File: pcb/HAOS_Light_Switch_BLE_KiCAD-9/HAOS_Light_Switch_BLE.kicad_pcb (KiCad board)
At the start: 2 copper layers, 30.1 x 29.9 mm, 38 parts, among them J1 GPIO, J2 GPIO, J3 GPIO, J4 Battery_CR2032, J5 PWR, J6 Conn_ARM_SWD_TagConnect_TC203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, J7 SWD, SW1 SW_Push, SW2 SW_Push, SW3 SW_Push, U1 nrf52832, Y1 Q13FC1350000400, Y3 ABM8-32.000MHZ-B2-T3

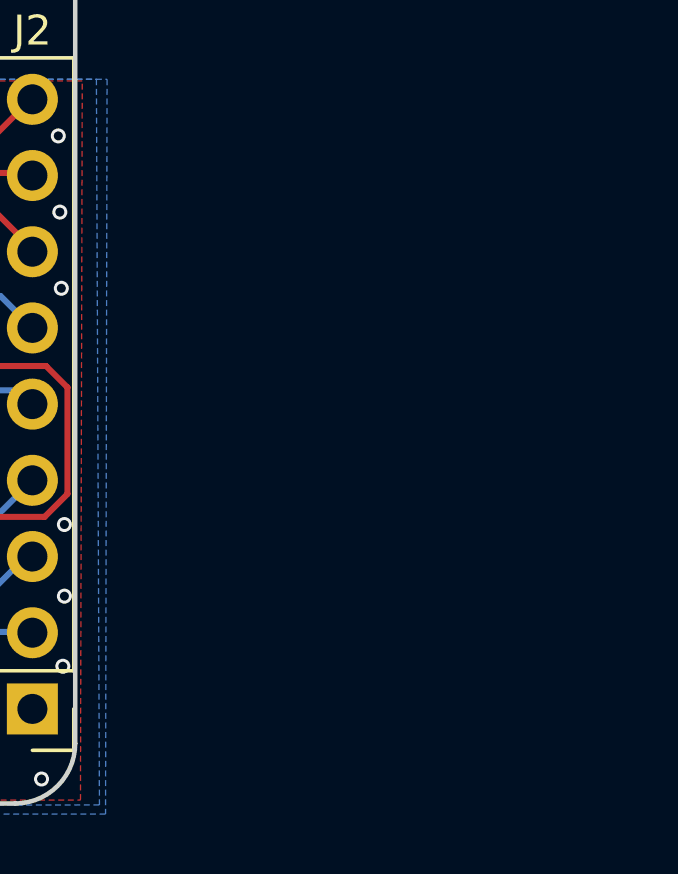
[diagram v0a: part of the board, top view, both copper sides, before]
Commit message: Draft AC power sniffer
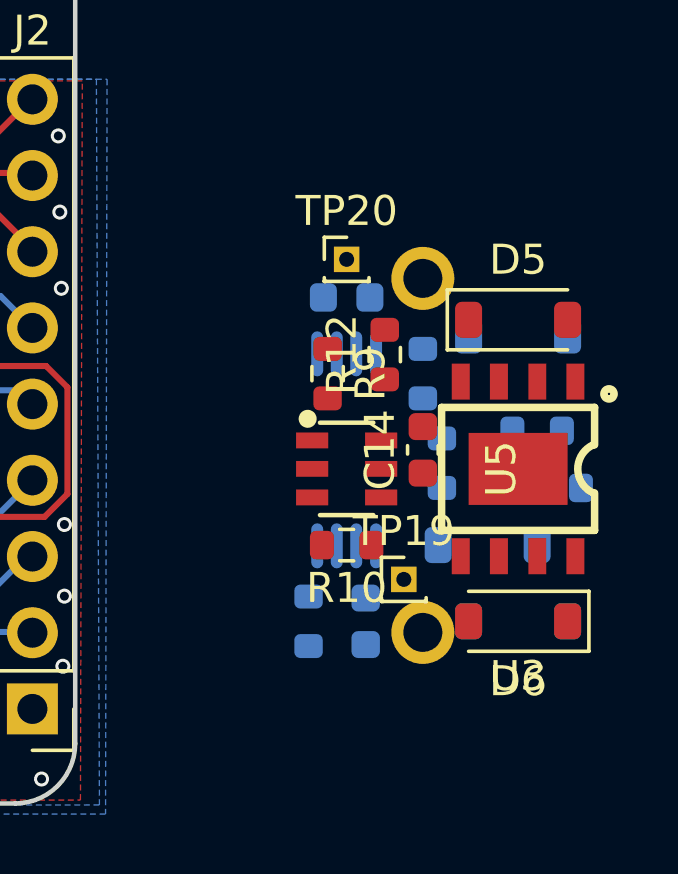
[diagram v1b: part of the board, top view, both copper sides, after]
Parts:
- added C14: 100n, Capacitor_SMD:C_0603_1608Metric, F.Cu at (205.1, 122.5)
- added C15: 10u, Capacitor_SMD:C_0603_1608Metric, B.Cu at (203.2, 128.2)
- added C16: 100n, Capacitor_SMD:C_0603_1608Metric, B.Cu at (202.6, 117.5)
- added D4: MBR0530, Diode_SMD:D_SOD-123, B.Cu at (207.3, 125.7)
- added D5: MBR0530, Diode_SMD:D_SOD-123, F.Cu at (208.3, 118.2)
- added D6: MBR0530, Diode_SMD:D_SOD-123, F.Cu at (208.3, 128.2)
- added D7: MBR0530, Diode_SMD:D_SOD-123, B.Cu at (208.3, 118.7)
- added D8: MBR0530, Diode_SMD:D_SOD-123, B.Cu at (208.3, 128.2)
- added R10: 0R, Resistor_SMD:R_0603_1608Metric, F.Cu at (202.6, 125.7)
- added R11: 100, Resistor_SMD:R_0603_1608Metric, B.Cu at (205.1, 120.0)
- added R12: 0R, Resistor_SMD:R_0603_1608Metric, F.Cu at (203.9, 119.4)
- added R5: 10K, Resistor_SMD:R_0603_1608Metric, B.Cu at (209.6, 123.8)
- added R6: 10K, Resistor_SMD:R_0603_1608Metric, B.Cu at (205.8, 123.0)
- added R7: 10K, Resistor_SMD:R_0603_1608Metric, B.Cu at (209.0, 121.9)
- added R8: 1K, Resistor_SMD:R_0603_1608Metric, B.Cu at (201.3, 128.2)
- added R9: 0R, Resistor_SMD:R_0603_1608Metric, F.Cu at (202.0, 120.0)
- added TP19: CONN_01, Connector_PinHeader_1.00mm:PinHeader_1x01_P1.00mm_Vertical, F.Cu at (204.5, 126.8)
- added TP20: CONN_01, Connector_PinHeader_1.00mm:PinHeader_1x01_P1.00mm_Vertical, F.Cu at (202.6, 116.2)
- added U2: ZMCT103C, easyeda2kicad:XFMR-TH_ZMCT103C, B.Cu at (205.1, 122.7)
- added U3: TP4056, easyeda2kicad:ESOP-8_L4.9-W3.9-P1.27-LS6.0-BL-EP, F.Cu at (208.3, 123.2)
- added U4: FS8205A, easyeda2kicad:TSSOP-8_L4.4-W3.0-P0.65-LS6.4-BL-2, B.Cu at (202.6, 122.5)
- added U5: DW01, easyeda2kicad:SOT-23-6_L2.9-W1.6-P0.95-LS2.8-BL, F.Cu at (202.6, 123.2)
